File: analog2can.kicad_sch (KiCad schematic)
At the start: 38 parts, among them J1 Conn_01x02_Socket, J2 DA15_Socket, J3 DT13-4P, J4 Conn_ARM_SWD_TagConnect_TC203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, U1 TJA1051T-E, U2 STM32U535CBTx, Y1 ABM8-16.000MHZ-D1X-T

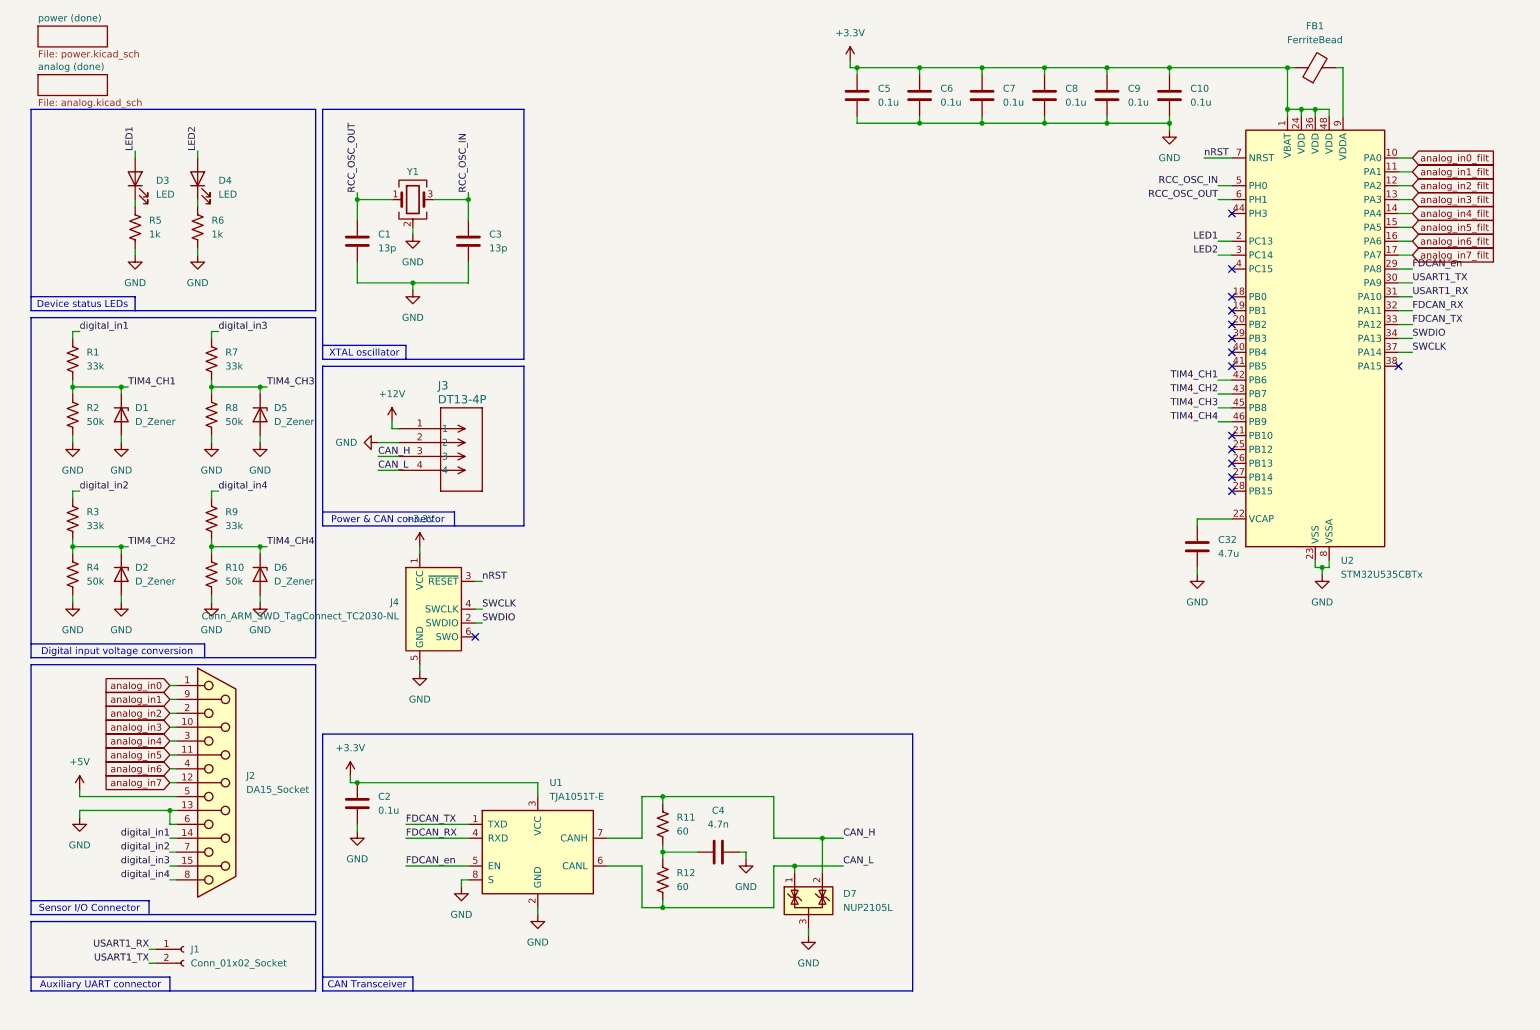
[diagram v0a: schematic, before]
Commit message: Debut layout PCB et review Schema done
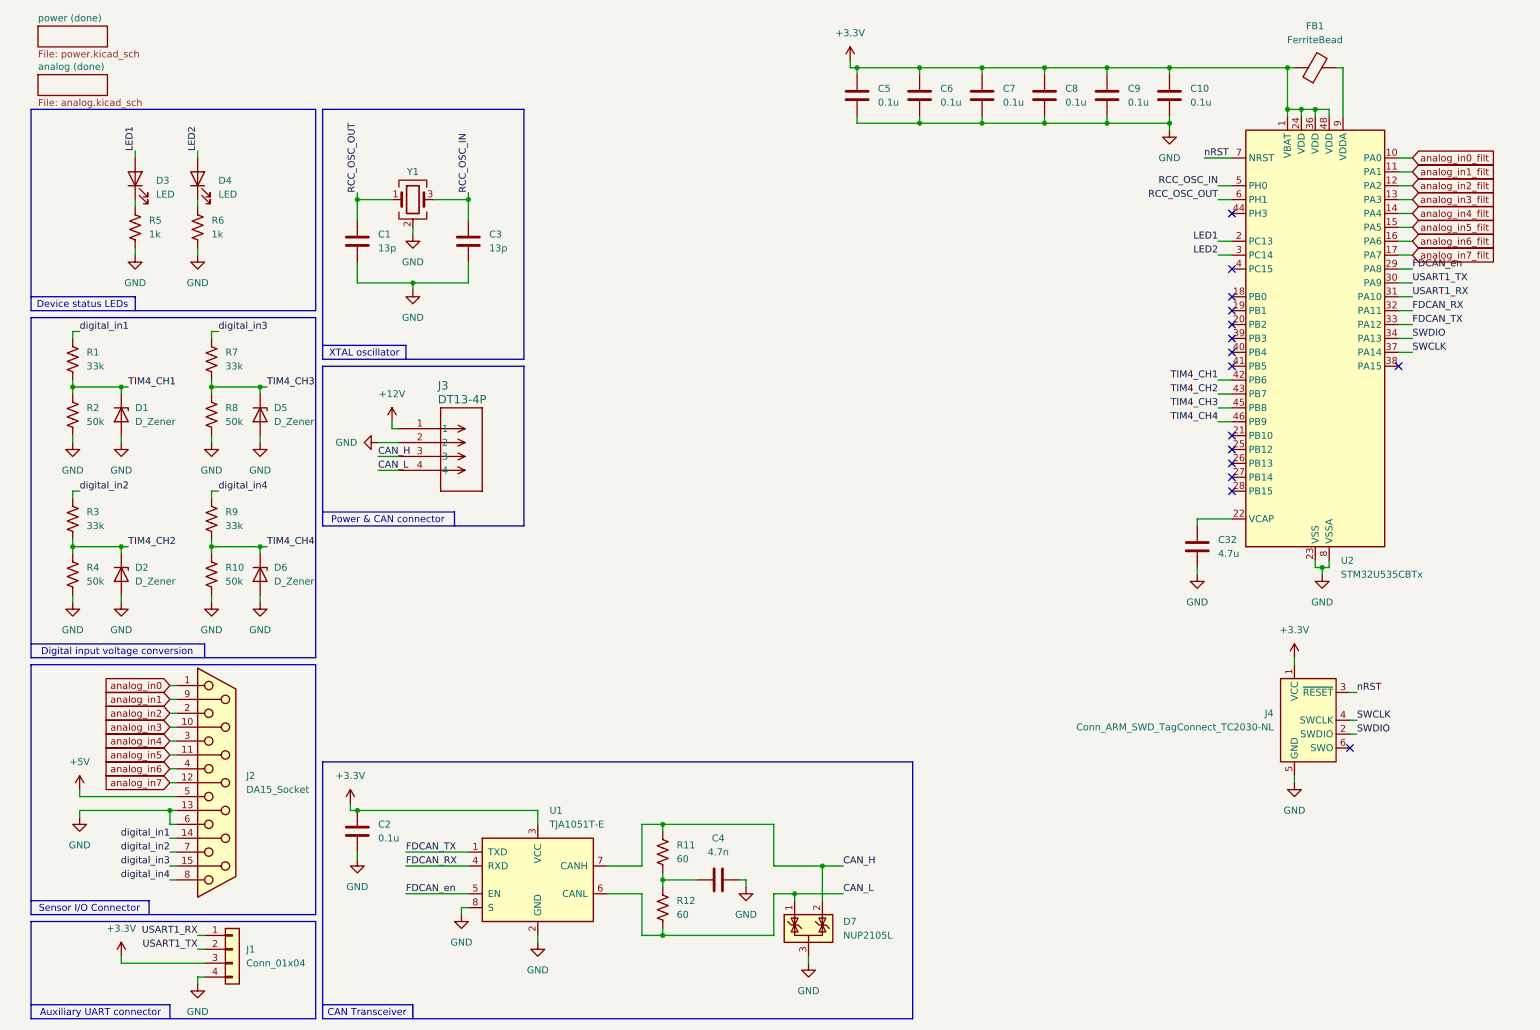
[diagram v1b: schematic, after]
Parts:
- removed J1: Conn_01x02_Socket, Connector_PinHeader_1.00mm:PinHeader_2x31_P1.00mm_Horizontal, symbol Connector:Conn_01x02_Socket
- added J1: Conn_01x04, Connector_Molex:Molex_KK-254_AE-6410-04A_1x04_P2.54mm_Vertical, symbol Connector_Generic:Conn_01x04
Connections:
- net +3.3V: now also J1.3 (Pin_3)
- net GND: now also J1.4 (Pin_4)
- net USART1_RX: now also J1.1 (Pin_1)
- net USART1_TX: now also J1.2 (Pin_2)
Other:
- moved on the sheet: C2, C4, D7, J4, R11, R12, U1
